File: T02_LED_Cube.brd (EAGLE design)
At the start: 61.9 x 80 mm, 43 parts, among them IC1 MSGEQ7SOIC, J1 POWER_JACKPTH, Q1 16MHz, Q2 IRF9530, Q3 IRF9530, Q4 IRF9530, U1 ATMEGA328P-AU, U2 TLC5940-RHB, U3 TLC5940-RHB, X1 1503_02

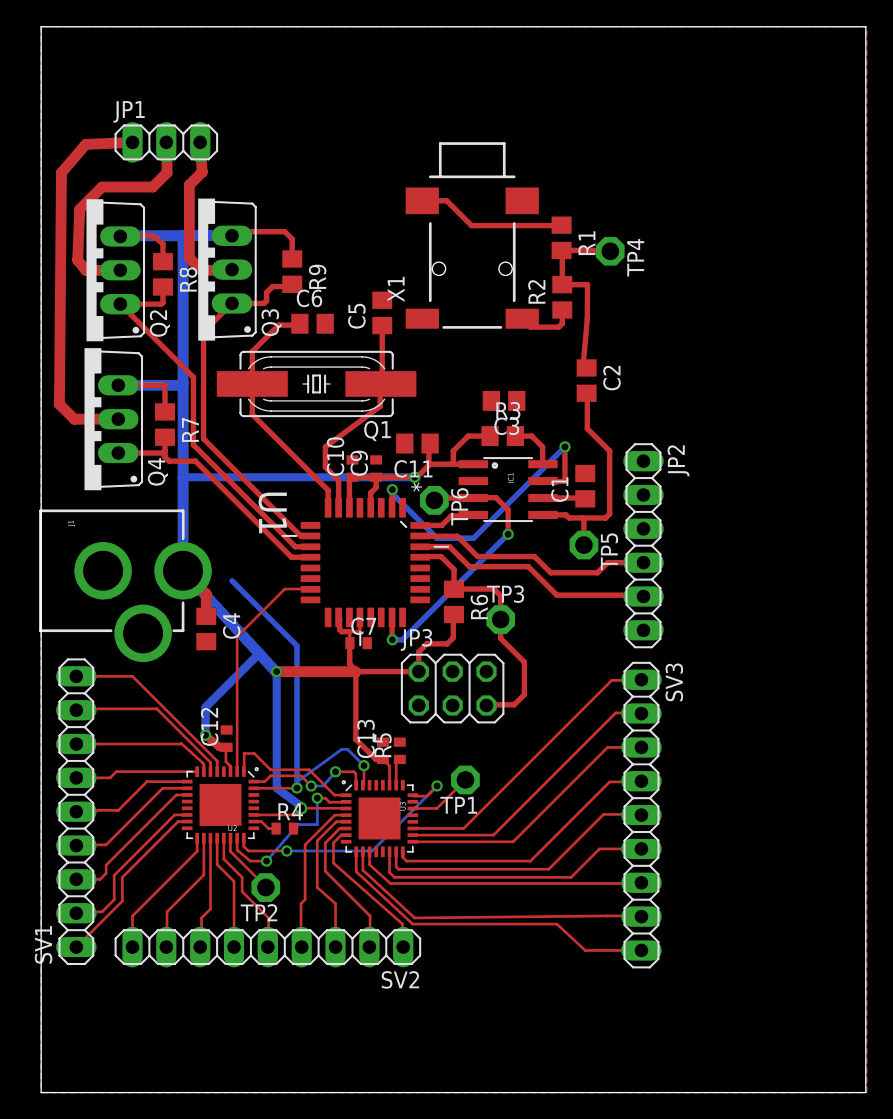
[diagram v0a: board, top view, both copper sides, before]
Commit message: pcb 75% done
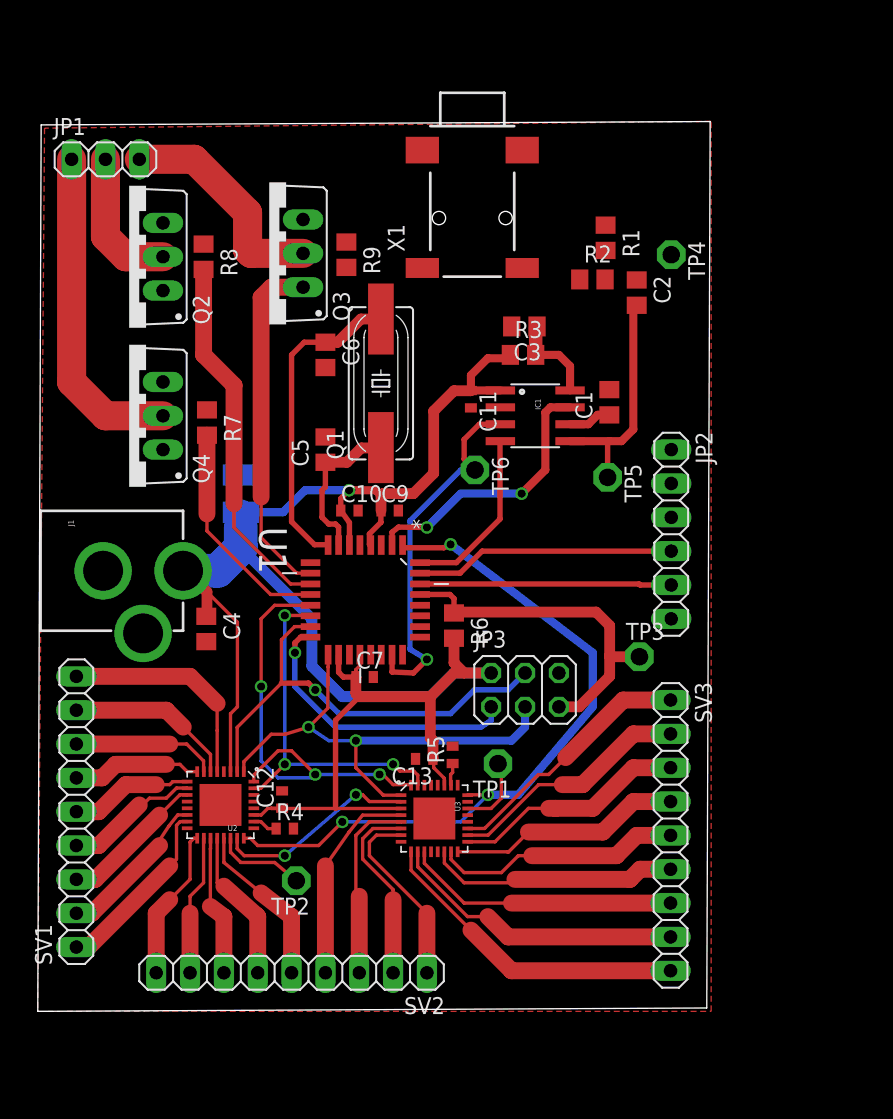
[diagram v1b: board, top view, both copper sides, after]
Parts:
- added R10: 0, rcl:R1210
- C10, C12, C13, C7, C9: value .1uF -> .15uF
- C11: value .1uF -> .15uF; device rcl:C0805 -> rcl:C0402
- moved C5 11.1 mm to (21.3, 48.3)
- moved TP3 10.8 mm to (44.9, 32.7)
- moved C2 7.60 mm to (44.7, 60.0)
- moved C1 6.55 mm to (42.6, 51.8)
- moved R3 6.28 mm to (36.2, 55.4)
- moved C12 6.19 mm to (18.1, 22.0)
- moved IC1 5.90 mm to (37.1, 50.8)
- moved C3 5.79 mm to (36.3, 57.5)
- moved Q3 5.47 mm to (17.1, 63.0)
- moved JP3 5.44 mm to (36.3, 30.2)
- moved TP5 5.38 mm to (42.5, 46.2)
- moved C11 5.21 mm to (32.3, 52.0), turned to 270 degrees
- moved Q1 4.83 mm to (25.5, 53.2), turned to 90 degrees
- moved JP1 4.75 mm to (4.83, 70.1)
- moved TP4 4.58 mm to (47.3, 62.9)
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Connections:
- net LAY4_SUPPLY renamed LAY1_SUPPLY
- net N$35 renamed SERIAL_TX
- new net LED_SUPPLY: Q2.S, Q3.S, Q4.S, R10.1, R7.1, R8.1, R9.1
- net +5V: now also R10.2; no longer Q2.S, Q3.S, Q4.S, R7.1, R8.1, R9.1
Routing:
- net TLC_GSCLK: track 19.4 -> 53.9 mm, vias 2 -> 3
- net +5V: track 170.9 -> 140.6 mm, vias 4 -> 2
- net SPI_SCLK: track 10.3 -> 37.4 mm, vias 0 -> 2
- net TLC_XLAT: track 9.57 -> 33.6 mm, vias 2 -> 3
- net SPI_MISO: track 0.00 -> 21.8 mm, vias 0 -> 1
- net SPI_MOSI: track 17.1 -> 34.4 mm, vias 0 -> 1
- net UNFILTERED_INPUT: track 14.5 -> 0.00 mm
- net N$2: track 11.8 -> 0.00 mm
- net MSG_STROBE: track 4.31 -> 13.2 mm
- net LAY3_SUPPLY: track 18.7 -> 10.7 mm
- net ATM_RST: track 19.5 -> 26.7 mm
- net MSG_OUT: track 21.5 -> 27.7 mm, vias 2 -> 1
- net LED14: track 8.69 -> 14.8 mm
- net CRY_2: track 18.5 -> 23.8 mm
- net CRY_1: track 16.2 -> 11.8 mm
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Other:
- board size 61.9 x 80 mm -> 50.5 x 66.8 mm

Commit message: board 95% besides stitching
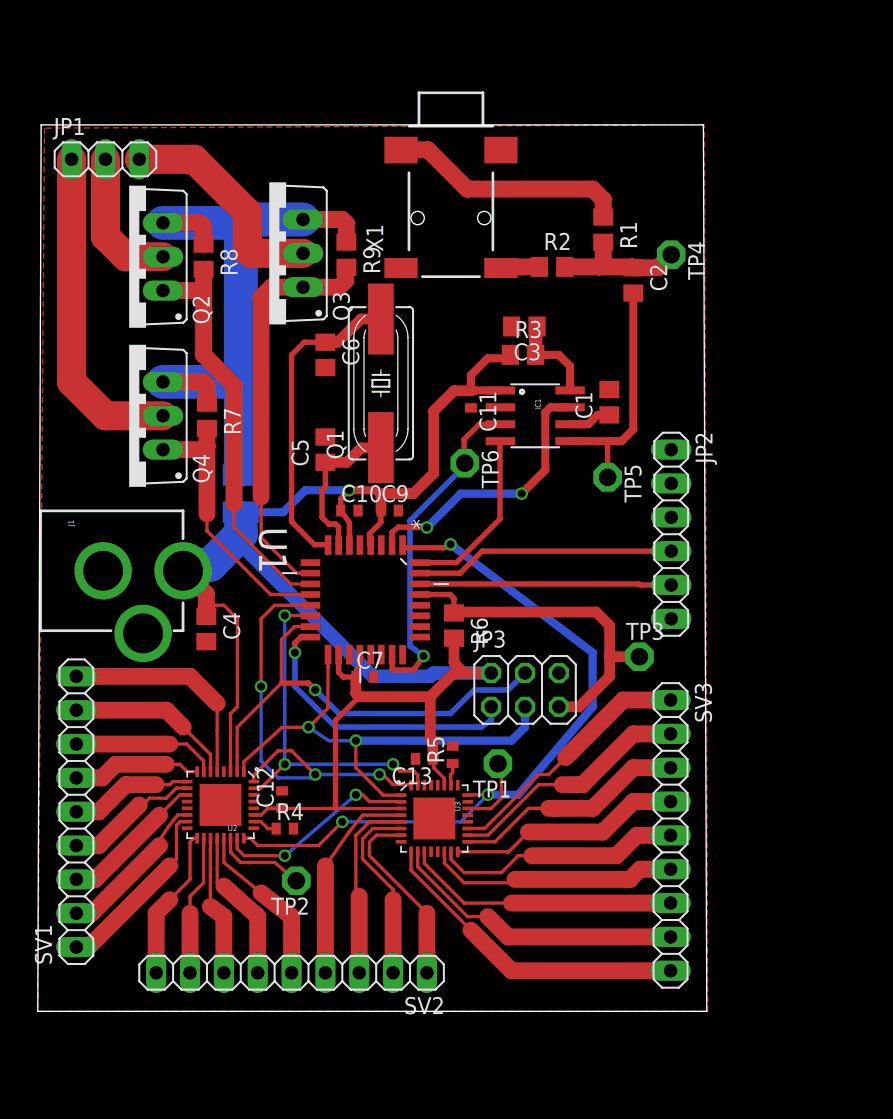
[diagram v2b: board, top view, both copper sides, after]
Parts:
- moved R2 3.17 mm to (38.4, 62.0)
- moved X1 1.60 mm to (30.8, 72.6)
- moved C2 0.95 mm to (44.5, 61.0)
- moved TP6 0.92 mm to (31.8, 47.2)
- moved R1 0.63 mm to (42.2, 64.8)
- moved R7 0.51 mm to (12.4, 50.8)
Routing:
- net LED_SUPPLY: track 0.00 -> 49.5 mm
- net N$2: track 0.00 -> 18.0 mm
- net UNFILTERED_INPUT: track 0.00 -> 10.4 mm
- net LAYER2_OFF: track 26.3 -> 30.7 mm
- net LAYER1_OFF: track 17.1 -> 21.1 mm
- net +5V: track 140.6 -> 137.1 mm, vias 2 -> 1
- net LAYER3_OFF: track 27.8 -> 31.0 mm
- net N$1: track 0.00 -> 2.93 mm
- net MSG_OUT: track 27.7 -> 25.7 mm
- net MSG_INPUT: track 17.3 -> 18.1 mm
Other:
- board size 50.5 x 66.8 mm -> 50.2 x 66.5 mm
